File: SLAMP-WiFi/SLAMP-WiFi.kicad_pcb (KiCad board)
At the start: 2 copper layers, 61.6 x 53.1 mm, 71 parts, among them P1 POWER_IN 5V, P11 GPIO15, P12 GPIO16, P2 USB_BUS, P3 VUSB, Q1 S8050, Q2 S8050, U1 MIC5219-3.3BM5, U2 CH340G, U4 TTP223, U5 TTP223, Y1 12 MHz

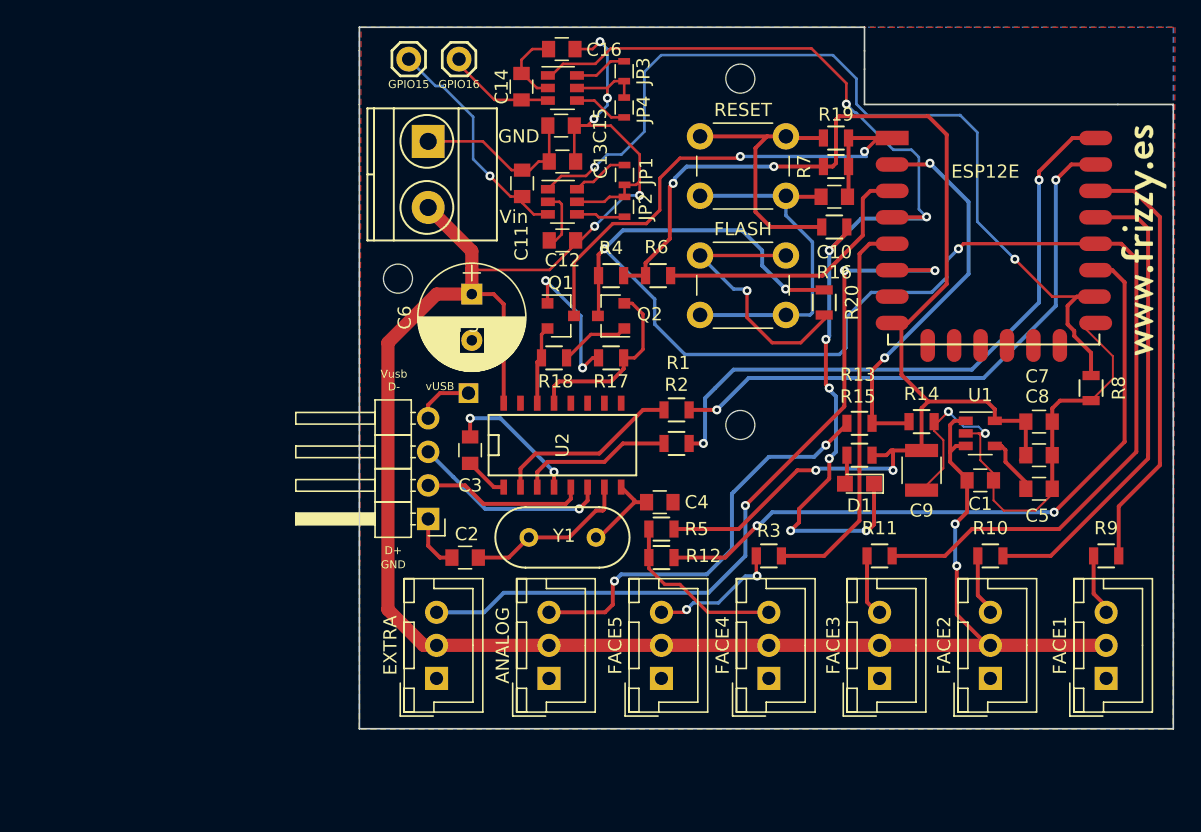
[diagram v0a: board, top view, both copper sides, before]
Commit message: placa ionut terminada
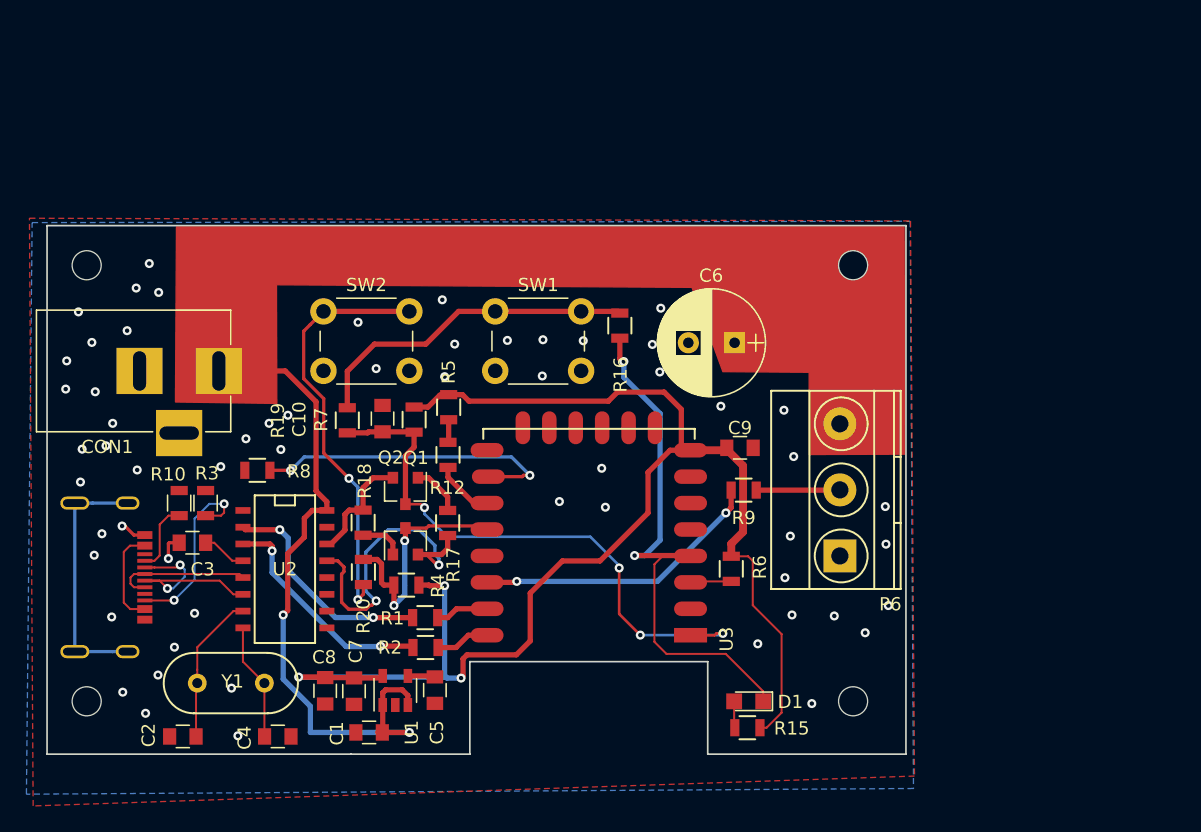
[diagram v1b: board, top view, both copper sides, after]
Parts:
- removed ANALOG: ADC, Connectors_JST:JST_XH_B03B-XH-A_03x2.50mm_Straight
- removed C11, C14: 30p, Capacitors_SMD:C_0805
- removed C12, C15: 100n, Capacitors_SMD:C_0805
- removed C13, C16: 10uF, Capacitors_SMD:C_0805
- removed ESP12E: ESP-12F, ESP8266:ESP-12E
- removed EXTRA: EXTRA, Connectors_JST:JST_XH_B03B-XH-A_03x2.50mm_Straight
- removed FACE1: FACE1, Connectors_JST:JST_XH_B03B-XH-A_03x2.50mm_Straight
- removed FACE2: FACE2, Connectors_JST:JST_XH_B03B-XH-A_03x2.50mm_Straight
- removed FACE3: FACE3, Connectors_JST:JST_XH_B03B-XH-A_03x2.50mm_Straight
- removed FACE4: FACE4, Connectors_JST:JST_XH_B03B-XH-A_03x2.50mm_Straight
- removed FACE5: FACE5, Connectors_JST:JST_XH_B03B-XH-A_03x2.50mm_Straight
- removed G***: LOGO, Grape:web
- removed G***: LOGO, logos_frizzy:logo_slamp_wifi_oro
- removed G***: LOGO, logos_frizzy:wifi_ola
- removed G***: LOGO, logos_frizzy:logo_wifi
- removed JP1, JP2, JP3, JP4: Jumper, Resistors_SMD:R_0603
- removed P1: POWER_IN 5V, Connectors_Terminal_Blocks:TerminalBlock_Pheonix_MKDS1.5-2pol
- removed P11: GPIO15, Connectors:1X01
- removed P12: GPIO16, Connectors:1X01
- removed P2: USB_BUS, Pin_Headers:Pin_Header_Angled_1x04_Pitch2.54mm
- removed P3: VUSB, Pin_Headers:Pin_Header_Straight_1x01
- removed R11: 470, Resistors_SMD:R_0805
- removed R13: 220k, Resistors_SMD:R_0805
- removed R14: 100k, Resistors_SMD:R_0805
- removed the REF** at (146.6, 74.0)
- removed the REF** at (172.5, 85.1)
- removed the REF** at (172.5, 58.9)
- removed REF***: OSHW-Symbol_6.7x6mm_SilkScreen, Symbols:OSHW-Symbol_6.7x6mm_SilkScreen
- removed U4, U5: TTP223, TO_SOT_Packages_SMD:SOT-23-6
- added CON1: POWER_IN_5V, Connectors:BARREL_JACK, F.Cu at (133.0, 81.0)
- added P6: FACE1, Connectors_Terminal_Blocks:TerminalBlock_Pheonix_MKDS1.5-3pol, F.Cu at (180.0, 95.0)
- added REF**: MountingHole_2.2mm_M2, Mounting_Holes:MountingHole_2.2mm_M2, F.Cu at (181.0, 106.0)
- added REF**: MountingHole_2.2mm_M2, Mounting_Holes:MountingHole_2.2mm_M2, F.Cu at (181.0, 73.0)
- added REF**: MountingHole_2.2mm_M2, Mounting_Holes:MountingHole_2.2mm_M2, F.Cu at (123.0, 73.0)
- added REF**: MountingHole_2.2mm_M2, Mounting_Holes:MountingHole_2.2mm_M2, F.Cu at (123.0, 106.0)
- added U3: ESP-12F, ESP8266:ESP-12E, F.Cu at (168.0, 101.0)
- added USB1: HRO-TYPE-C-31-M-12, Type-C:HRO-TYPE-C-31-M-13, F.Cu at (120.0, 96.6)
- C9: footprint Capacitors_SMD:C_1210 -> Capacitors_SMD:C_0805
- R10, R3: value 470 -> 5k1
- moved R8 63.4 mm to (135.9, 88.5), turned to 180 degrees
- moved R10 61.5 mm to (130.0, 91.0), turned to 90 degrees
- moved C8 56.9 mm to (141.0, 105.2), turned to 270 degrees
- moved C7 55.7 mm to (143.2, 105.2), turned to 270 degrees
- moved C1 50.0 mm to (144.4, 108.4), turned to 180 degrees
- moved U1 48.4 mm to (146.4, 105.2), turned to 90 degrees
- moved C5 48.2 mm to (149.4, 105.2), turned to 270 degrees
- moved R3 42.8 mm to (132.0, 91.0), turned to 90 degrees
- moved R19 42.7 mm to (142.7, 84.7), turned to 90 degrees
- moved R20 40.4 mm to (143.9, 96.2)
- moved C10 38.1 mm to (145.4, 84.6), turned to 90 degrees
- moved R7 37.2 mm to (147.8, 84.7), turned to 90 degrees
- moved C4 33.9 mm to (137.5, 108.7)
- moved SW2 28.8 mm to (140.9, 76.5)
- moved R4 28.1 mm to (147.2, 97.2)
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- renumbered RESET to SW1, FLASH to SW2
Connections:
- R10 pad 1: FACE2 -> Net-(R10-Pad1)
- R10 pad 2: Net-(R10-Pad2) -> GND
- R3 pad 2: FACE5 -> GND
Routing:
- net GND: track 98.9 -> 3.98 mm, vias 2 -> 60
- net GPIO0: track 112.2 -> 18.8 mm, vias 3 -> 2
- net EXTRA: track 59.2 -> 0.00 mm, vias 3 -> 0
- net 5V: track 172.2 -> 115.1 mm, vias 7 -> 2
- net Net-(R12-Pad2): track 53.1 -> 5.21 mm, vias 2 -> 0
- net GPIO15: track 68.0 -> 23.3 mm
- net RXD: track 47.5 -> 4.79 mm, vias 2 -> 0
- net GPIO16: track 83.3 -> 41.3 mm, vias 8 -> 2
- net TXD: track 43.3 -> 4.71 mm, vias 2 -> 0
- net Net-(R10-Pad2): track 36.5 -> 0.00 mm
- net ANALOG: track 31.9 -> 0.00 mm, vias 2 -> 0
- net ADC: track 29.3 -> 0.00 mm, vias 2 -> 0
- net Net-(USB1-Pad13): track 0.00 -> 19.2 mm
- net EN: track 21.8 -> 3.81 mm
- net Net-(C11-Pad1): track 17.6 -> 0.00 mm, vias 1 -> 0
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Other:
- board size 61.6 x 53.1 mm -> 65 x 40 mm
- board text added: "5V"
- board text added: "DOUT"
- board text removed: "D+"
- board text removed: "D-"
- board text removed: "Vin"
- board text removed: "Vusb"
- board text removed: "vUSB"
